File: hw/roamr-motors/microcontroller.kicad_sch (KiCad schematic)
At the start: 1 part, among them U3 ESP32-S3-WROOM-1

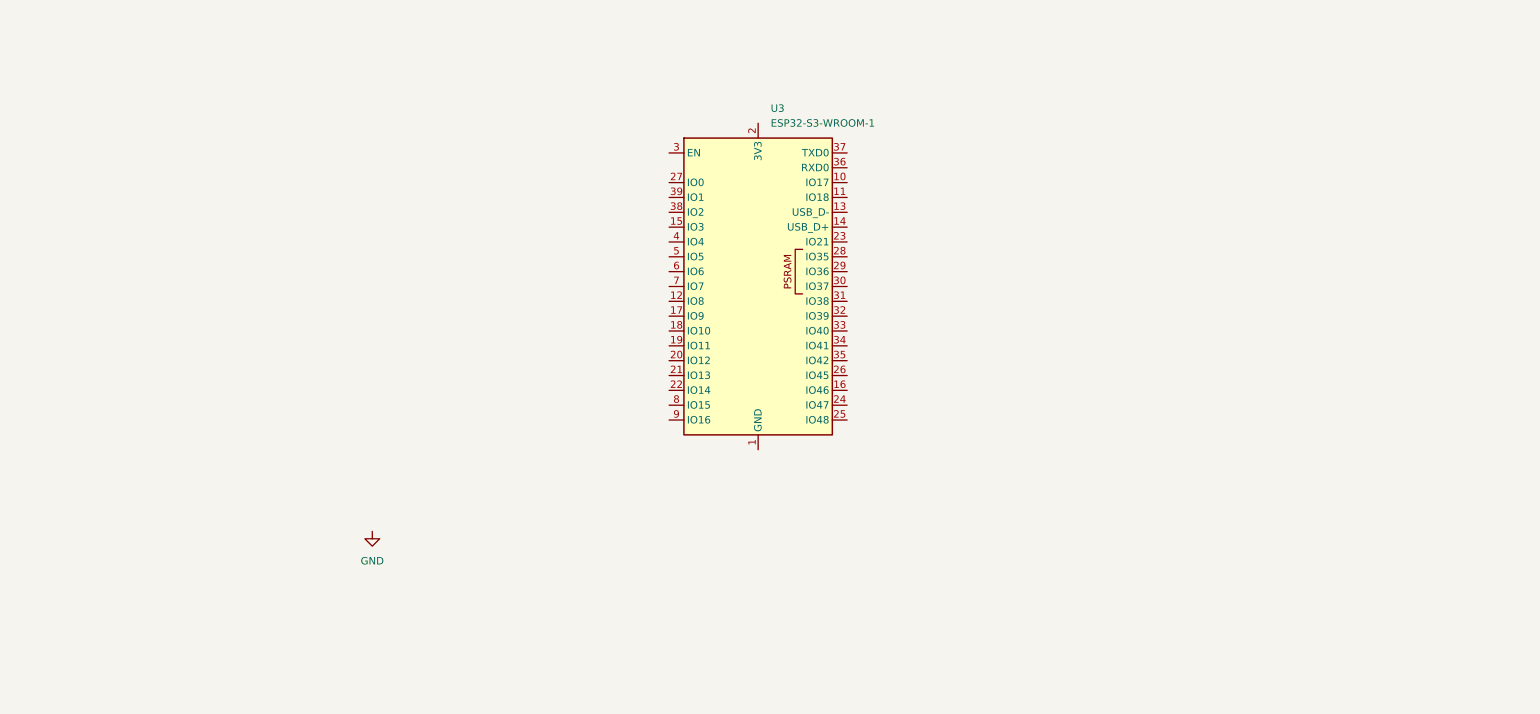
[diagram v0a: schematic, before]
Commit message: WIP ESP32 and USB UART
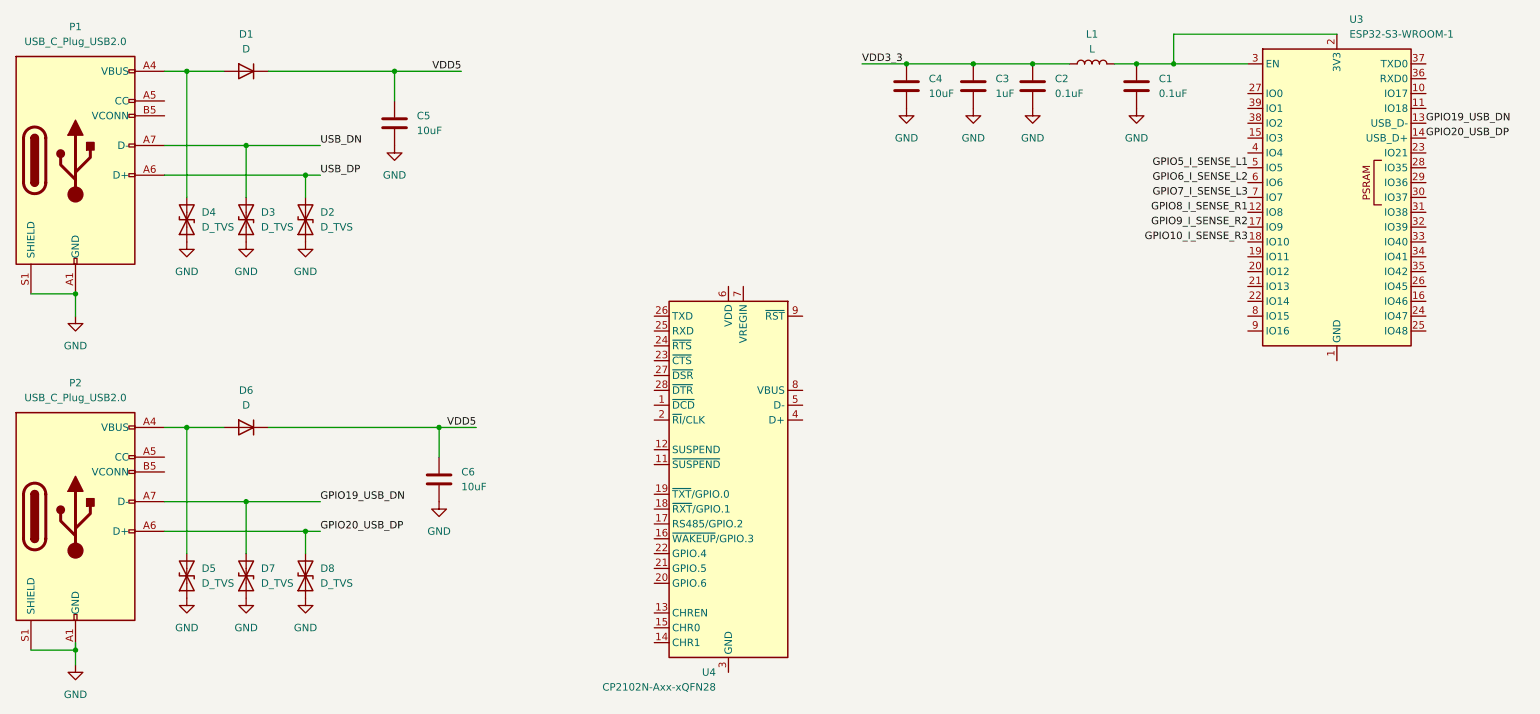
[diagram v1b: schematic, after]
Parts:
- added C1, C2: 0.1uF, symbol Device:C
- added C3: 1uF, symbol Device:C
- added C4, C5, C6: 10uF, symbol Device:C
- added D1, D6: D, symbol Device:D
- added D2, D3, D4, D5, D7, D8: D_TVS, symbol Device:D_TVS
- added L1: L, symbol Device:L
- added P1, P2: USB_C_Plug_USB2.0, symbol Connector:USB_C_Plug_USB2.0
- added U4: CP2102N-Axx-xQFN28, Package_DFN_QFN:QFN-28-1EP_5x5mm_P0.5mm_EP3.35x3.35mm, symbol Interface_USB:CP2102N-Axx-xQFN28
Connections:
- net GND: now also C1.2, C2.2, C3.2, C4.2, C5.2, C6.2, D2.1 (A1), D3.1 (A1), D4.1 (A1), D5.1 (A1), D7.1 (A1), D8.1 (A1), P1.A1 (GND), P1.A12 (GND), P1.B1 (GND), P1.B12 (GND), P1.S1 (SHIELD), P2.A1 (GND), P2.A12 (GND), P2.B1 (GND), P2.B12 (GND), P2.S1 (SHIELD)
- net GPIO8_I_SENSE_R1: now reaches U3.12 (IO8)
- net GPIO19_USB_DN: now reaches U3.13 (USB_D-)
- net GPIO19_USB_DN: now also D7.2 (A2), P2.A7 (D-)
- net GPIO20_USB_DP: now reaches U3.14 (USB_D+)
- net GPIO20_USB_DP: now also D8.2 (A2), P2.A6 (D+)
- net GPIO9_I_SENSE_R2: now reaches U3.17 (IO9)
- net GPIO10_I_SENSE_R3: now reaches U3.18 (IO10)
- net at U3.2 (3V3): now also U3.3 (EN), C1.1, L1.2
- net GPIO5_I_SENSE_L1: now reaches U3.5 (IO5)
- net GPIO6_I_SENSE_L2: now reaches U3.6 (IO6)
- net GPIO7_I_SENSE_L3: now reaches U3.7 (IO7)
- new net: D5.2 (A2), D6.2 (A), P2.A4 (VBUS), P2.A9 (VBUS), P2.B4 (VBUS), P2.B9 (VBUS)
- new net: D1.2 (A), D4.2 (A2), P1.A4 (VBUS), P1.A9 (VBUS), P1.B4 (VBUS), P1.B9 (VBUS)
- new net: U4.29 (GND), U4.3 (GND)
- new net USB_DN: D3.2 (A2), P1.A7 (D-)
- new net USB_DP: D2.2 (A2), P1.A6 (D+)
- new net VDD3_3: C2.1, C3.1, C4.1, L1.1
- new net VDD5: C5.1, C6.1, D1.1 (K), D6.1 (K)
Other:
- moved on the sheet: U3
